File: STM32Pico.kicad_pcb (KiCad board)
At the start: 2 copper layers, 21.1 x 51.3 mm, 25 parts, among them J1 2.54mm header 01x20, J2 2.54mm header 01x20, SW1 Boot Mode, SW2 Reset Switch, U1 STM32F411CEUx, U2 XC6206PxxxMR, X1 ECS-2520MV-xxx-xx

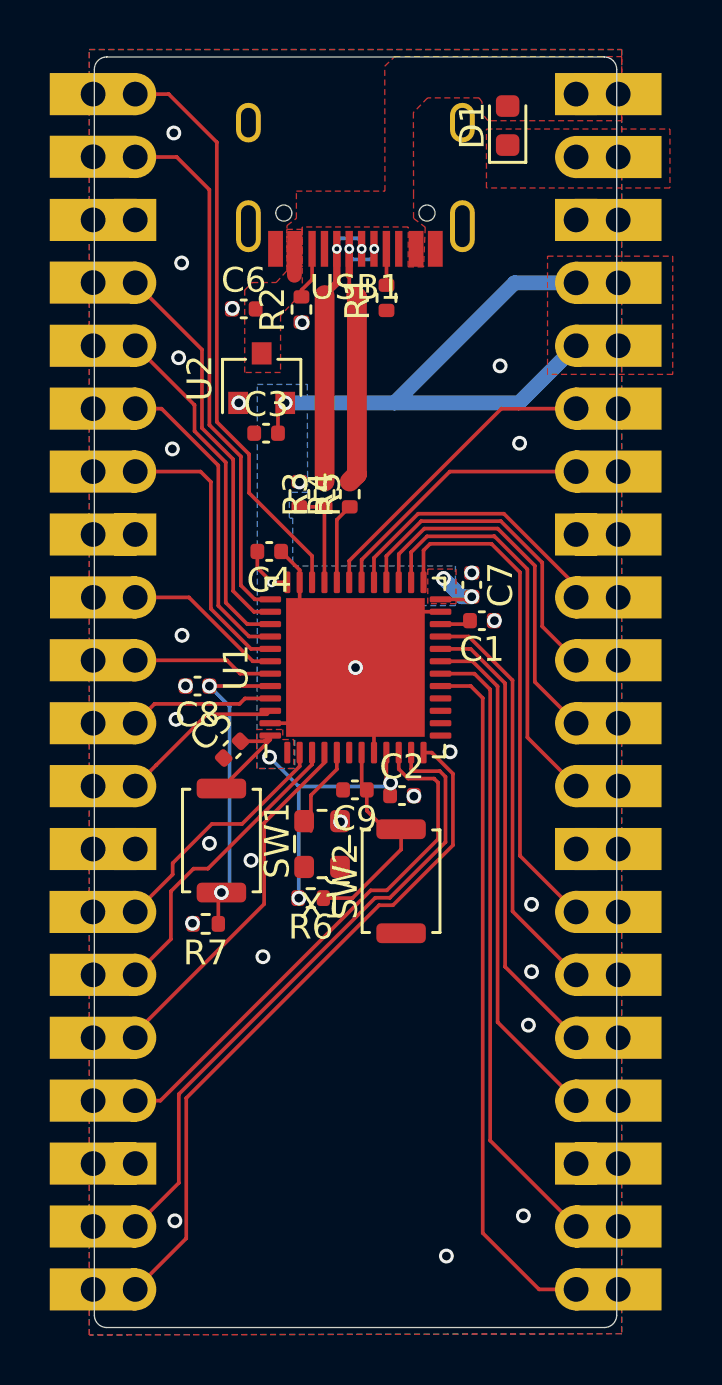
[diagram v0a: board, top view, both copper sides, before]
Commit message: cleaned up some bits and pieces.
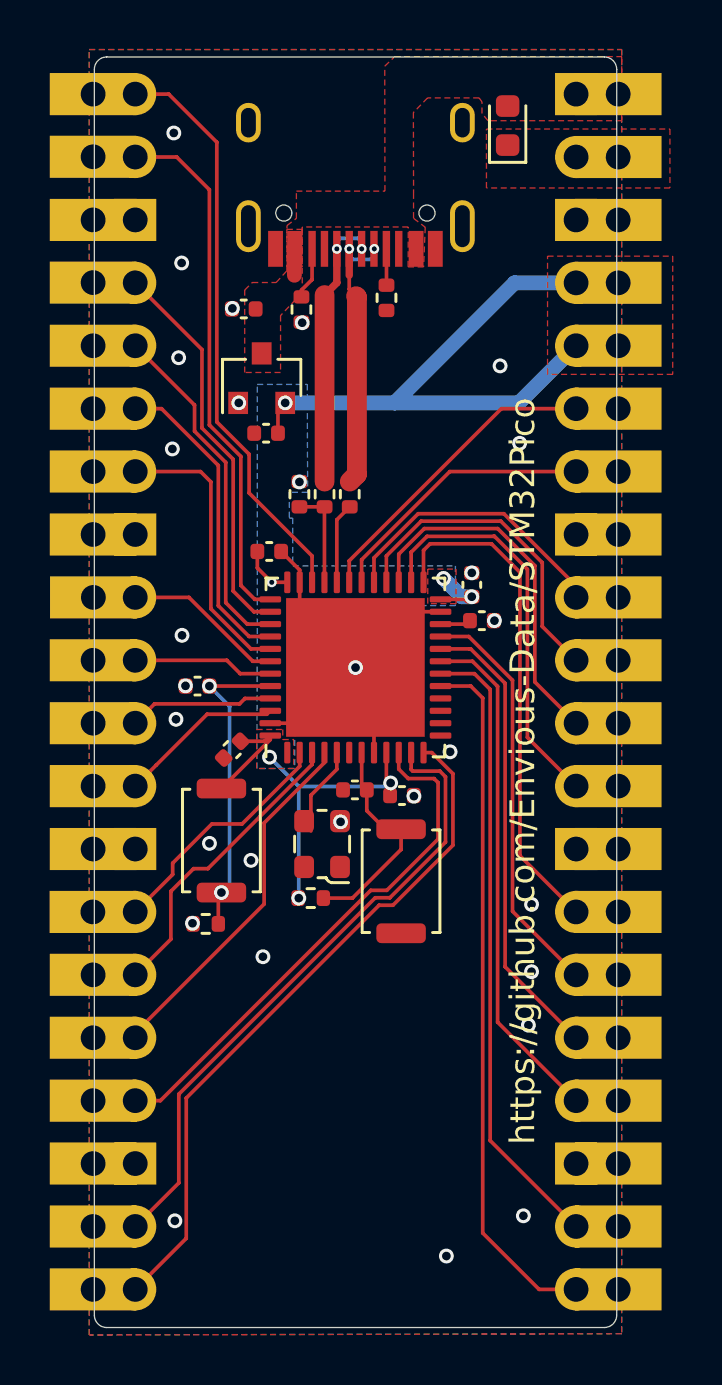
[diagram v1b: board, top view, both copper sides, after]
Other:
- board text added: "https://github.com/Envious-Data/STM32Pico"
